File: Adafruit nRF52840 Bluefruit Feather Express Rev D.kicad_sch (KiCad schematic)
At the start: 41 parts, among them IC2 GD25Q16, J1 USB_C_Receptacle_USB2.0, Q3 DMG2305, SW101 KMR2, SW102 KMR2, U0 USBLC6-2SC6, U2 AP2112(3.3V), U3 MCP73831T-2ACI/OT, X3 JSTPH, Y2 32.768

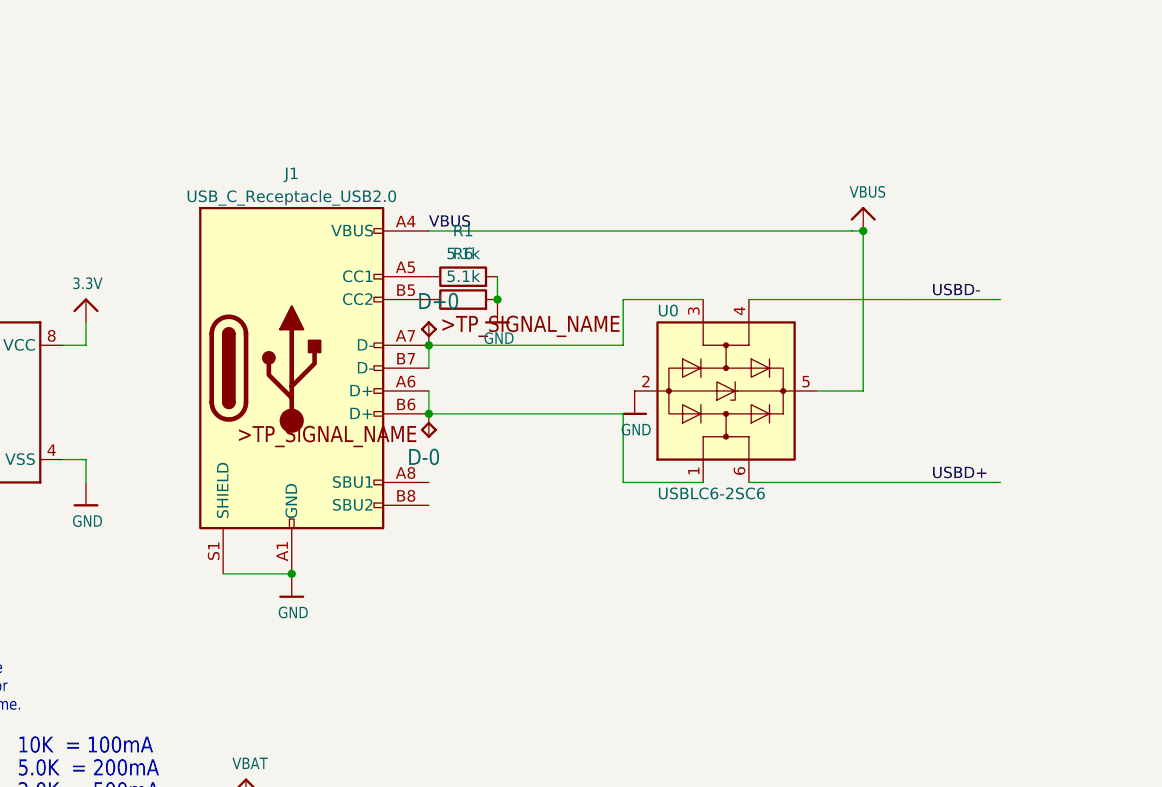
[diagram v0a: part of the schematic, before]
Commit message: Small work
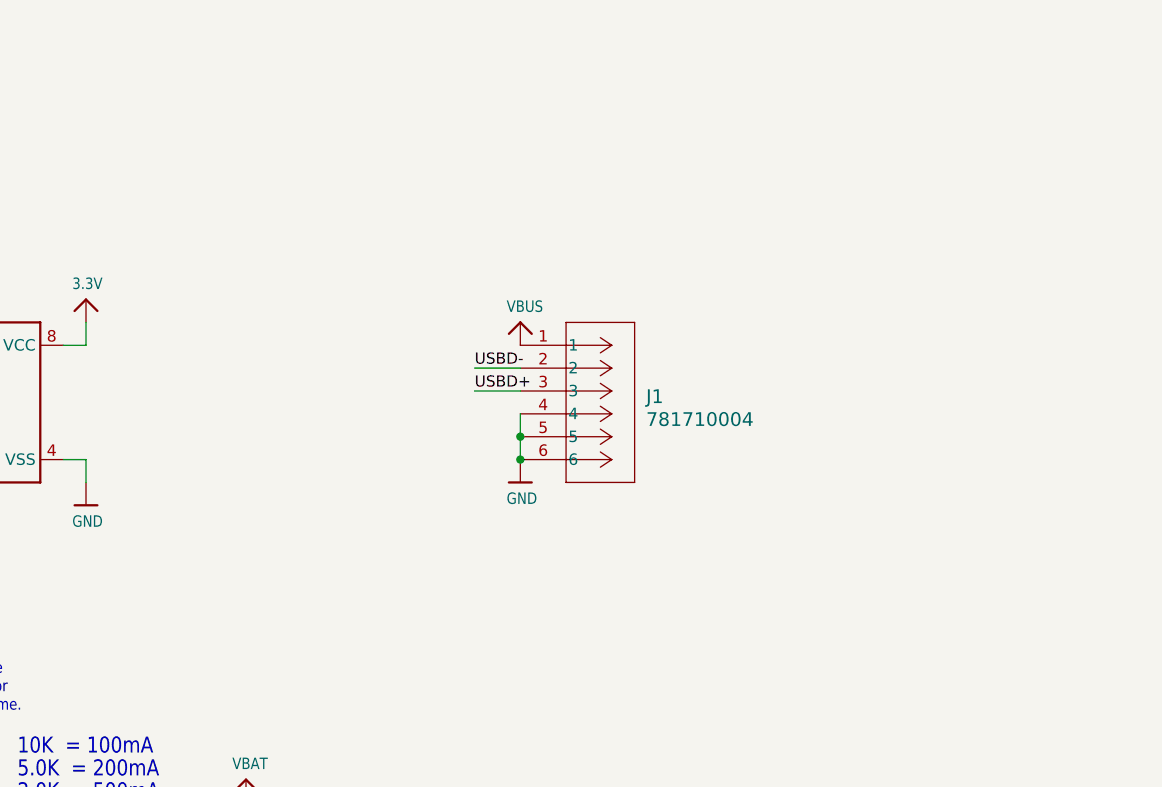
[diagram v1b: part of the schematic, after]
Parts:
- removed D+0, D-0: TPTP10R, Adafruit nRF52840 Bluefruit Feather Express Rev D:TP10R, symbol Adafruit nRF52840 Bluefruit Feather Express Rev D-eagle-import:TPTP10R
- removed J1: USB_C_Receptacle_USB2.0, JohnDeereLibrary:GCT USB4510-03-1-A, symbol Connector:USB_C_Receptacle_USB2.0
- removed R1, R6: 5.1k, Resistor_SMD:R_0603_1608Metric, symbol Device:R
- removed U0: USBLC6-2SC6, Package_TO_SOT_SMD:SOT-23-6, symbol Power_Protection:USBLC6-2SC6
- added J1: 781710004, CON_781710004, symbol 2023-09-18_17-26-43:781710004
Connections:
- net GND: now also J1.4, J1.5, J1.6
- net USBD+: now also J1.3
- net USBD-: now also J1.2
- net VBUS: now also J1.1
